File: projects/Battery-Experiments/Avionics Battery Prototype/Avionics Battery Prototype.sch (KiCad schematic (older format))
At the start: 21 parts, among them U1 LM324A

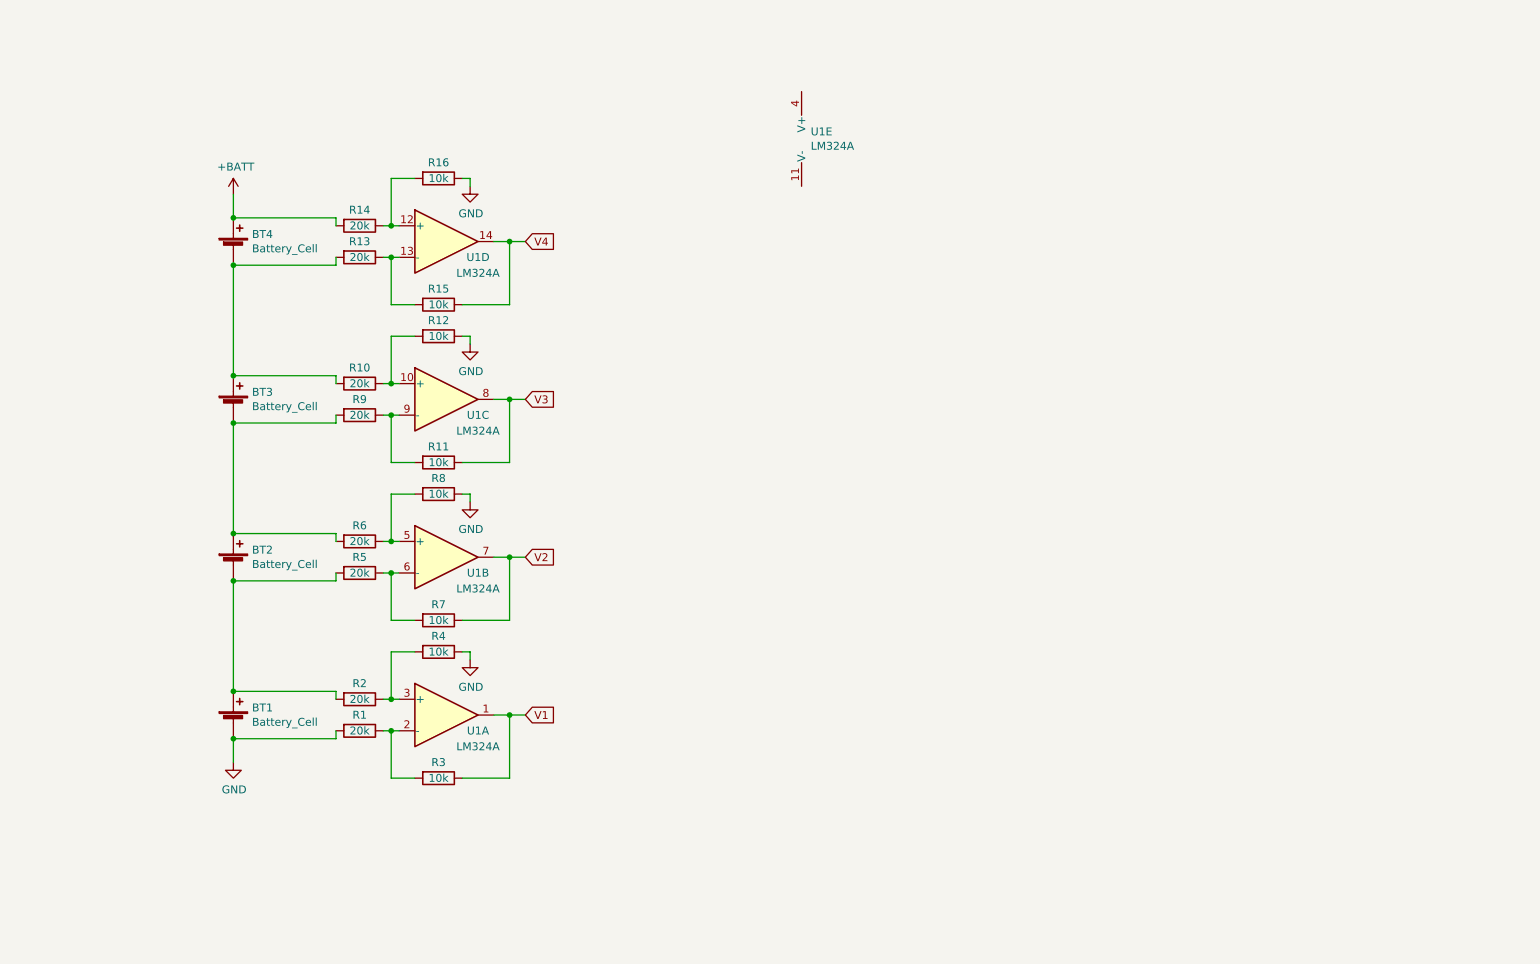
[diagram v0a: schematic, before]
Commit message: AVB Start
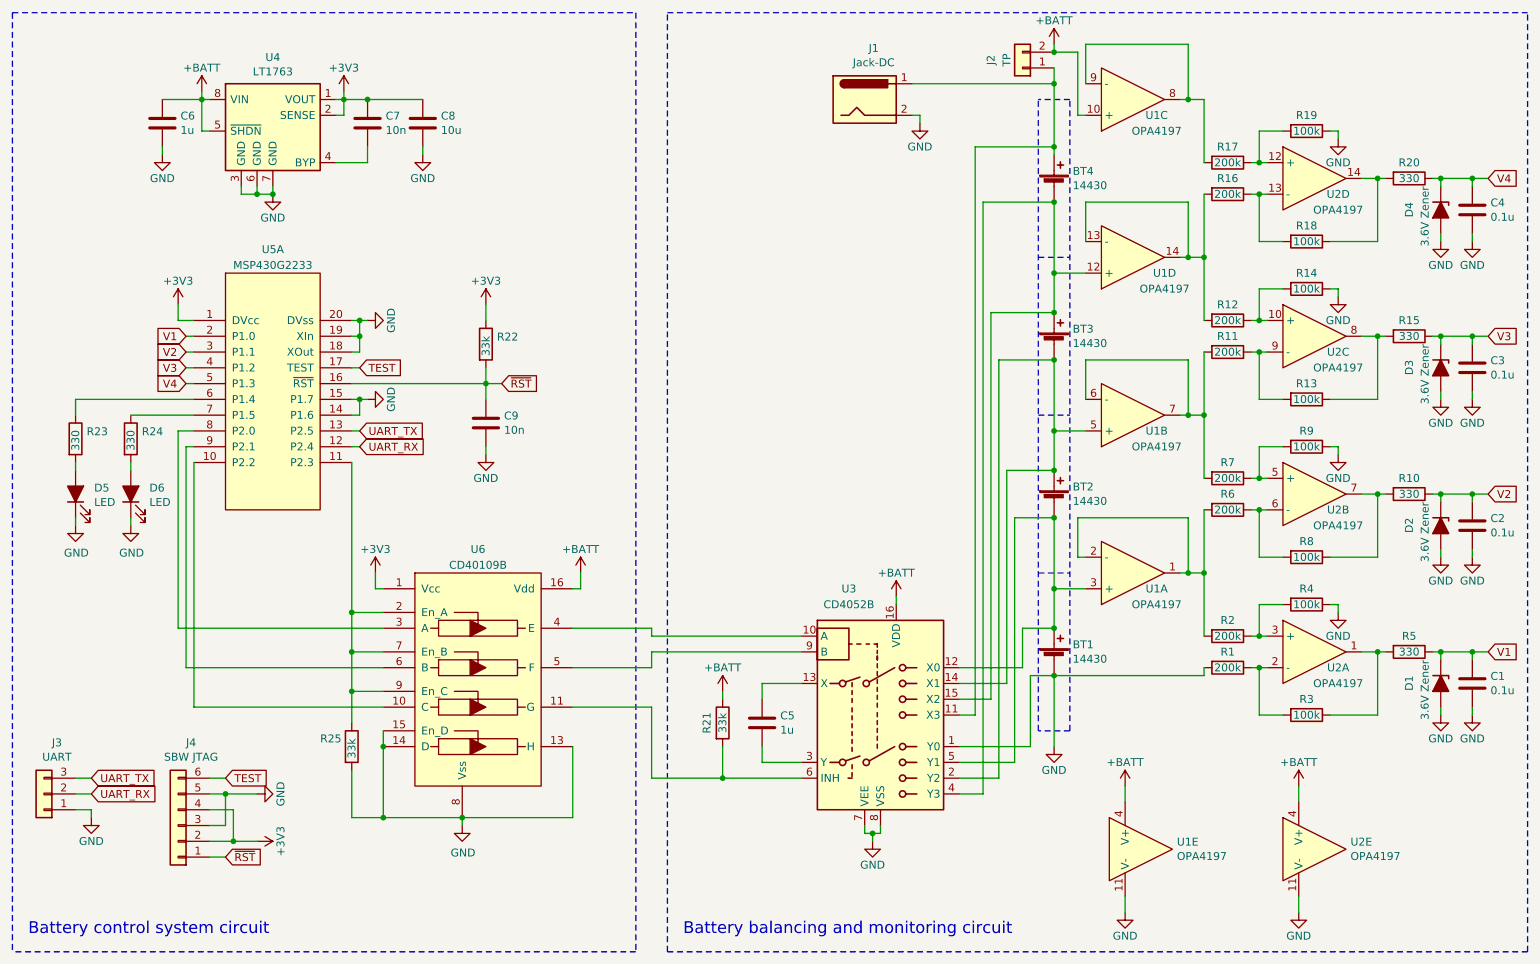
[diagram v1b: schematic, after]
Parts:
- removed U1: LM324A, symbol Amplifier_Operational:LM324A
- added C1, C2, C3, C4: 0.1u, Capacitors_SMD:C_1206_HandSoldering, symbol Device:C
- added C5, C6: 1u, Capacitors_SMD:C_1206_HandSoldering, symbol Device:C
- added C7, C9: 10n, Capacitors_SMD:C_1206_HandSoldering, symbol Device:C
- added C8: 10u, Capacitors_SMD:C_1206_HandSoldering, symbol Device:C
- added D1, D2, D3, D4: 3.6V Zener, Diodes_SMD:D_SOD-123F, symbol Device:D_Zener_ALT
- added D5, D6: LED, LEDs:LED_1206_HandSoldering, symbol Device:LED_ALT
- added J1: Jack-DC, Connect:Banana_Jack_2Pin, symbol Connector:Jack-DC
- added J2: TP, Pin_Headers:Pin_Header_Straight_1x02_Pitch2.54mm, symbol Connector_Generic:Conn_01x02
- added J3: UART, Pin_Headers:Pin_Header_Straight_1x03_Pitch2.54mm, symbol Connector_Generic:Conn_01x03
- added J4: SBW JTAG, Pin_Headers:Pin_Header_Straight_1x06_Pitch2.54mm, symbol Connector_Generic:Conn_01x06
- added R10, R15, R20, R23, R24, R5: 330, Resistors_SMD:R_1206_HandSoldering, symbol Device:R
- added R21, R22, R25: 33k, Resistors_SMD:R_1206_HandSoldering, symbol Device:R
- added U1, U2: OPA4197, SMD_Packages:SOIC-14_N, symbol k7arx:OPA4322
- added U3: CD4052B, SMD_Packages:SO-16-N, symbol Analog_Switch:CD4052B
- added U4: LT1763, SMD_Packages:SOIC-8-N, symbol k7arx:LT1763
- added U5: MSP430G2233, SMD_Packages:SSOP-20, symbol k7arx:MSP430G2233
- added U6: CD40109B, SMD_Packages:SO-16-N, symbol k7arx:CD40109B
- BT1, BT2, BT3, BT4: value Battery_Cell -> 14430; footprint (none) -> k7arx:Keystone-92 Battery_Contact 14430
- R1, R2: value 20k -> 200k; footprint (none) -> Resistors_SMD:R_1206_HandSoldering
- R11: renamed from R9; value 20k -> 200k; footprint (none) -> Resistors_SMD:R_1206_HandSoldering
- R12: renamed from R10; value 20k -> 200k; footprint (none) -> Resistors_SMD:R_1206_HandSoldering
- R13: renamed from R11; value 10k -> 100k; footprint (none) -> Resistors_SMD:R_1206_HandSoldering
- R14: renamed from R12; value 10k -> 100k; footprint (none) -> Resistors_SMD:R_1206_HandSoldering
- R16: renamed from R13; value 20k -> 200k; footprint (none) -> Resistors_SMD:R_1206_HandSoldering
- R17: renamed from R14; value 20k -> 200k; footprint (none) -> Resistors_SMD:R_1206_HandSoldering
- R18: renamed from R15; value 10k -> 100k; footprint (none) -> Resistors_SMD:R_1206_HandSoldering
- R19: renamed from R16; value 10k -> 100k; footprint (none) -> Resistors_SMD:R_1206_HandSoldering
- R3, R4: value 10k -> 100k; footprint (none) -> Resistors_SMD:R_1206_HandSoldering
- R6: renamed from R5; value 20k -> 200k; footprint (none) -> Resistors_SMD:R_1206_HandSoldering
- R7: renamed from R6; value 20k -> 200k; footprint (none) -> Resistors_SMD:R_1206_HandSoldering
- R8: renamed from R7; value 10k -> 100k; footprint (none) -> Resistors_SMD:R_1206_HandSoldering
- R9: renamed from R8; value 10k -> 100k; footprint (none) -> Resistors_SMD:R_1206_HandSoldering
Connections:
- net +BATT: now also C6.1, J2.2 (Pin_2), R21.1, U1.10 (+), U1.4 (V+), U2.4 (V+), U3.16 (VDD), U4.5 (~SHDN), U4.8 (VIN), U6.16 (Vdd); no longer BT4.1 (+), R17.2
- net GND: now also C1.2, C2.2, C3.2, C4.2, C6.2, C8.2, C9.2, D1.2 (A), D2.2 (A), D3.2 (A), D4.2 (A), D5.1 (K), D6.1 (K), J1.2, J3.1 (Pin_1), J4.3 (Pin_3), J4.5 (Pin_5), R25.2, U1.11 (V-), U2.11 (V-), U3.1 (Y0), U3.7 (VEE), U3.8 (VSS), U4.3 (GND), U4.6 (GND), U4.7 (GND), U5.14 (P1.6), U5.15 (P1.7), U5.18 (XOut), U5.19 (XIn), U5.20 (DVss), U6.13 (H), U6.14 (D), U6.15 (En_D), U6.8 (Vss)
- net V1: now also C1.1, D1.1 (K), R5.1, U5.2 (P1.0); no longer R3.1
- net V2: now also C2.1, D2.1 (K), R10.1, U5.3 (P1.1); no longer R8.1
- net V3: now also C3.1, D3.1 (K), R15.1, U5.4 (P1.2); no longer R13.1
- net V4: now also C4.1, D4.1 (K), R20.1, U5.5 (P1.3); no longer R18.1
- net at BT3.1 (+), BT4.2 (-): now also U1.12 (+), U3.15 (X2), U3.4 (Y3); no longer R12.2, R16.2
- net at BT2.1 (+), BT3.2 (-): now also U1.5 (+), U3.14 (X1), U3.2 (Y2); no longer R11.2, R7.2
- net at BT1.1 (+), BT2.2 (-): now also U1.3 (+), U3.12 (X0), U3.5 (Y1); no longer R2.2, R6.2
- net at R1.1, R3.2: now also U2.2 (-)
- net at R2.1, R4.2: now also U2.3 (+)
- net at R7.1, R9.2: now also U2.5 (+)
- net at R6.1, R8.2: now also U2.6 (-)
- net at R12.1, R14.2: now also U2.10 (+)
- net at R11.1, R13.2: now also U2.9 (-)
- net at R17.1, R19.2: now also U2.12 (+)
- net at R16.1, R18.2: now also U2.13 (-)
- new net: BT4.1 (+), J1.1, J2.1 (Pin_1), U3.11 (X3)
- new net: R2.2, R6.2, U1.1, U1.2 (-)
- new net: R11.2, R7.2, U1.6 (-), U1.7
- new net: R12.2, R16.2, U1.13 (-), U1.14
- new net: R17.2, U1.8, U1.9 (-)
- new net: C5.1, U3.13 (X)
- new net: C5.2, U3.3 (Y)
- new net: U3.10 (A), U6.4 (E)
- new net: R21.2, U3.6 (INH), U6.11 (G)
- new net: U3.9 (B), U6.5 (F)
- new net: R3.1, R5.2, U2.1
- new net: R10.2, R8.1, U2.7
- new net: R13.1, R15.2, U2.8
- new net: R18.1, R20.2, U2.14
- new net: C7.2, U4.4 (BYP)
- new net: U5.10 (P2.2), U6.10 (C)
- new net: R25.1, U5.11 (P2.3), U6.2 (En_A), U6.7 (En_B), U6.9 (En_C)
- new net: U5.8 (P2.0), U6.3 (A)
- new net: U5.9 (P2.1), U6.6 (B)
- new net: R23.1, U5.6 (P1.4)
- new net: D5.2 (A), R23.2
- new net: R24.1, U5.7 (P1.5)
- new net: D6.2 (A), R24.2
- new net +3V3: C7.1, C8.1, J4.2 (Pin_2), J4.4 (Pin_4), R22.1, U4.1 (VOUT), U4.2 (SENSE), U5.1 (DVcc), U6.1 (Vcc)
- new net TEST: J4.6 (Pin_6), U5.17 (TEST)
- new net UART_RX: J3.2 (Pin_2), U5.12 (P2.4)
- new net UART_TX: J3.3 (Pin_3), U5.13 (P2.5)
- new net ~RST: C9.1, J4.1 (Pin_1), R22.2, U5.16 (~RST)
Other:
- note added: "Battery balancing and monitoring circuit"
- note added: "Battery control system circuit"
- moved on the sheet: BT1, BT2, BT3, BT4, R1, R11, R12, R13, R14, R16, R17, R18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
